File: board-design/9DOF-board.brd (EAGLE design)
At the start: 100 x 80 mm, 0 parts

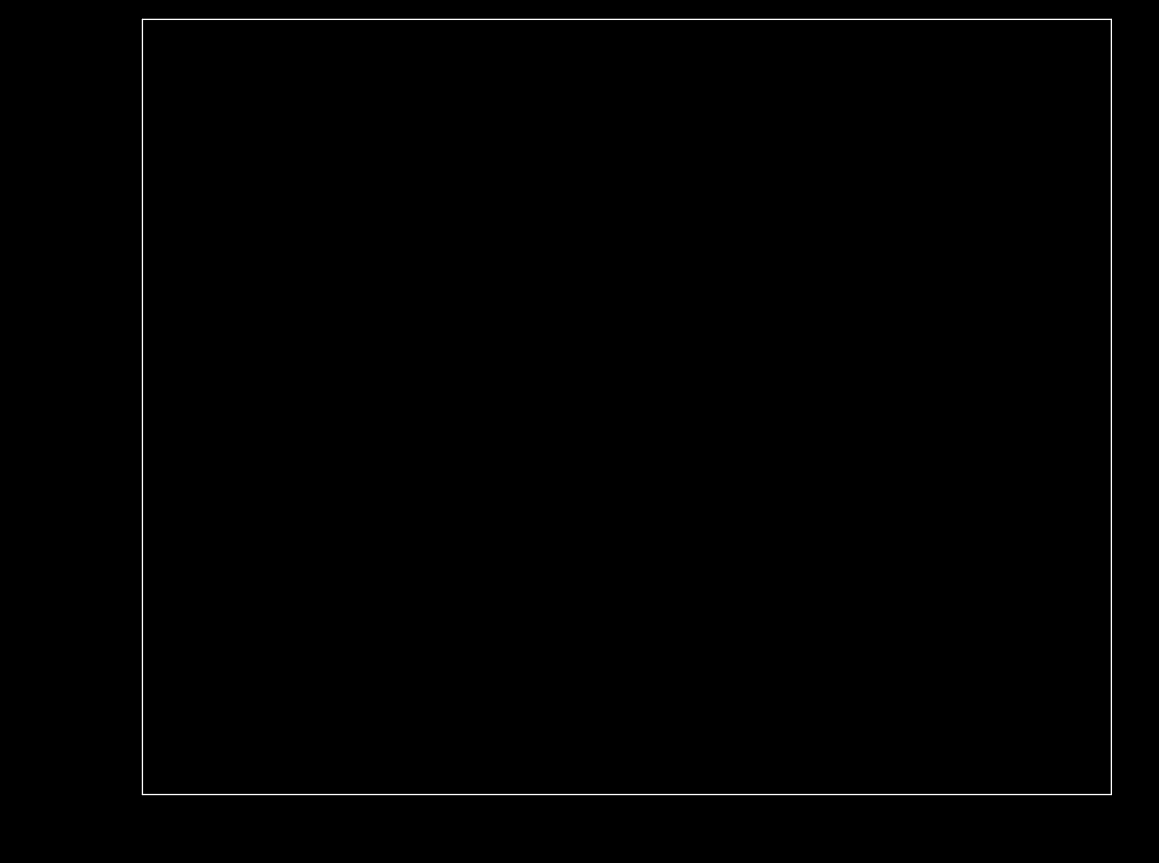
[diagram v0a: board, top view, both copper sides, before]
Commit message: Add files via upload
PCB Layout v0.1
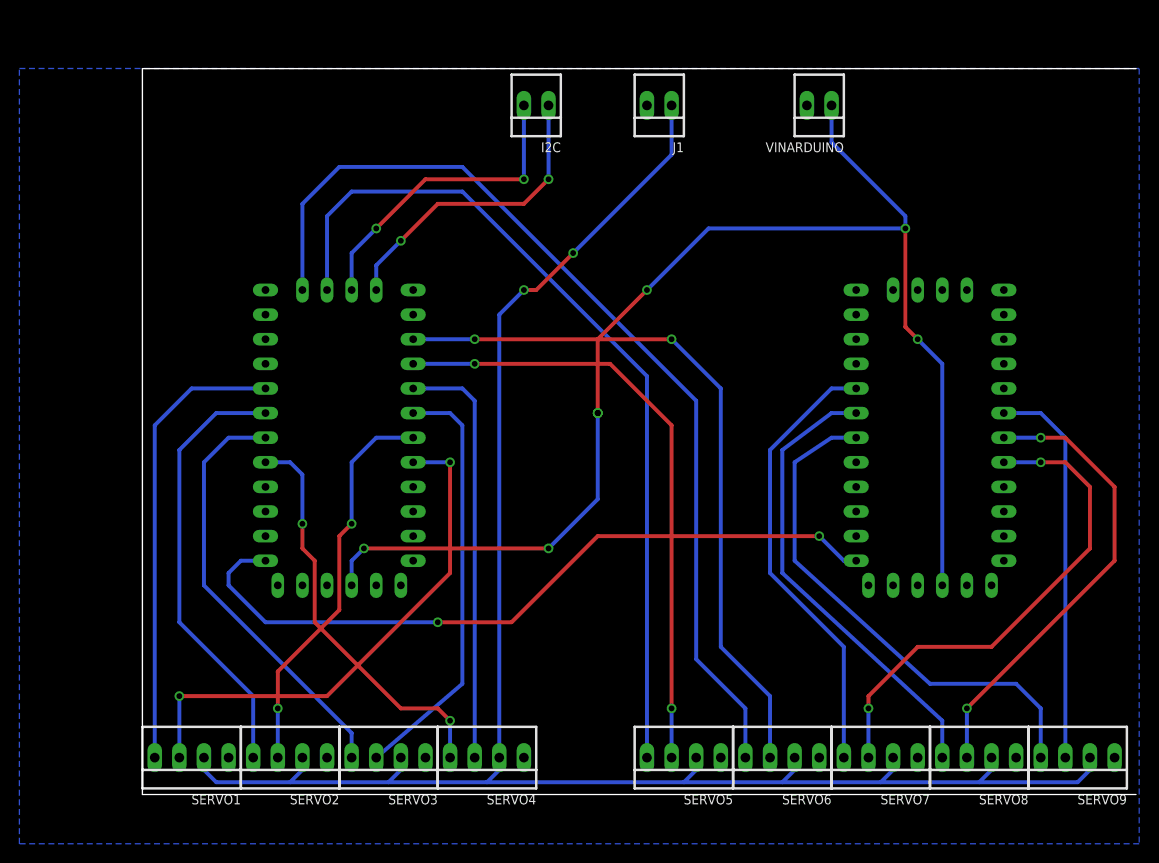
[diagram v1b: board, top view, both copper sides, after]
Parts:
- added I2C, J1, VINARDUINO: (no value), con-molex:22-23-2021
- added SERVO1, SERVO2, SERVO3, SERVO4, SERVO5, SERVO6, SERVO7, SERVO8, SERVO9: 22-23-2041, con-molex:22-23-2041
- added U$1, U$2: PRO-MINI, Arduino-clone:PRO-MINI
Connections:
- new net GND: J1.2, SERVO1.1, SERVO2.1, SERVO3.1, SERVO4.1, SERVO5.1, SERVO6.1, SERVO7.1, SERVO8.1, SERVO9.1, U$1.GND, U$1.GND3, U$2.GND, U$2.GND3, VINARDUINO.2
- new net I2C_SCA: I2C.1, U$1.A4
- new net I2C_SCL: I2C.2, U$1.A5
- new net RAW: U$1.RAW, U$2.RAW
- new net SERVO1_POT: SERVO1.4, U$1.A0
- new net SERVO1_SIG: SERVO1.3, U$1.D2
- new net SERVO2_POT: SERVO2.4, U$1.A1
- new net SERVO2_SIG: SERVO2.3, U$1.D3
- new net SERVO3_POT: SERVO3.4, U$1.A2
- new net SERVO3_SIG: SERVO3.3, U$1.D4
- new net SERVO4_POT: SERVO4.4, U$1.A3
- new net SERVO4_SIG: SERVO4.3, U$1.D5
- new net SERVO5_POT: SERVO5.4, U$1.A6
- new net SERVO5_SIG: SERVO5.3, U$1.D6
- new net SERVO6_POT: SERVO6.4, U$1.A7
- new net SERVO6_SIG: SERVO6.3, U$1.D7
- new net SERVO7_POT: SERVO7.4, U$2.A0
- new net SERVO7_SIG: SERVO7.3, U$2.D2
- new net SERVO8_POT: SERVO8.4, U$2.A1
- new net SERVO8_SIG: SERVO8.3, U$2.D3
- new net SERVO9_POT: SERVO9.4, U$2.A2
- new net SERVO9_SIG: SERVO9.3, U$2.D4
- new net VCC_ARDUINO: U$1.VCC1, U$2.VCC1, VINARDUINO.1
- new net VCC_SERVO: J1.1, SERVO1.2, SERVO2.2, SERVO3.2, SERVO4.2, SERVO5.2, SERVO6.2, SERVO7.2, SERVO8.2, SERVO9.2
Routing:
- net VCC_SERVO: track 0.00 -> 191.9 mm, vias 0 -> 2
- net VCC_ARDUINO: track 0.00 -> 137.8 mm, vias 0 -> 8
- net SERVO6_POT: track 0.00 -> 100.0 mm
- net SERVO5_POT: track 0.00 -> 89.0 mm
- net RAW: track 0.00 -> 76.7 mm, vias 0 -> 2
- net SERVO6_SIG: track 0.00 -> 74.1 mm, vias 0 -> 2
- net SERVO5_SIG: track 0.00 -> 63.6 mm, vias 0 -> 2
- net SERVO1_SIG: track 0.00 -> 54.8 mm, vias 0 -> 2
- net SERVO9_POT: track 0.00 -> 53.7 mm
- net SERVO7_SIG: track 0.00 -> 51.8 mm, vias 0 -> 2
- net SERVO8_POT: track 0.00 -> 47.9 mm
- net SERVO8_SIG: track 0.00 -> 47.8 mm, vias 0 -> 2
- net SERVO1_POT: track 0.00 -> 47.3 mm
- net SERVO7_POT: track 0.00 -> 46.4 mm
- net SERVO2_POT: track 0.00 -> 45.4 mm
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- added copper zone on layer 16, net GND
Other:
- board size 100 x 80 mm -> 102.5 x 74.9 mm
